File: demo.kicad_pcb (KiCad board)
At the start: 4 copper layers, 36 x 12.5 mm, 32 parts, among them J2 Conn_01x06, J3 Conn_01x04, J4 USB_C_Receptacle, U1 Regulator_Linear_XC6220B331MR, U2 MCU_ST_STM32F1_STM32F103C8Tx, Y2 8M

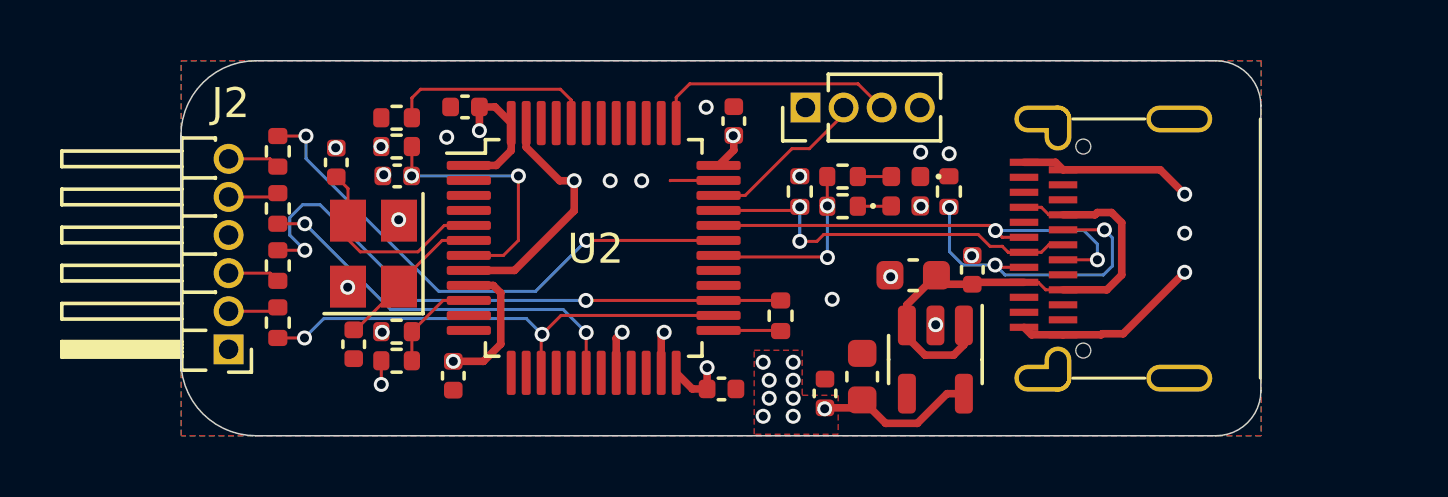
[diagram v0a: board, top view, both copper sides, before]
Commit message: update files
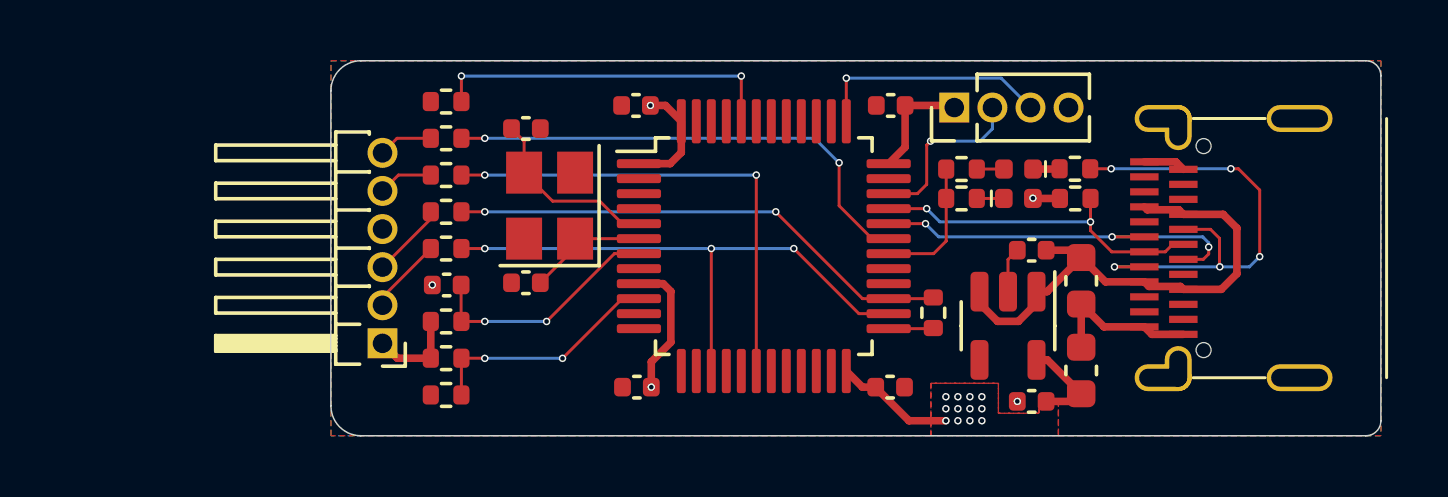
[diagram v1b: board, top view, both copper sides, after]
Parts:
- moved C5 17.0 mm to (118.6, 110.9), turned to 0 degrees
- moved C3 11.0 mm to (118.7, 101.5), turned to 180 degrees
- moved R8 9.18 mm to (124.8, 104.6), turned to 0 degrees
- moved C7 7.30 mm to (125.0, 110.3)
- moved C8 6.90 mm to (123.4, 111.4), turned to 180 degrees
- moved C10 6.42 mm to (106.5, 102.3), turned to 180 degrees
- moved C4 6.13 mm to (110.2, 110.9), turned to 180 degrees
- moved R4 6.13 mm to (103.8, 106.3), turned to 180 degrees
- moved C9 6.10 mm to (106.5, 107.4), turned to 0 degrees
- moved Y2 6.08 mm to (107.3, 104.8)
- moved R11 6.06 mm to (103.8, 108.7)
- moved R5 5.89 mm to (103.8, 105.0), turned to 180 degrees
- moved R6 5.72 mm to (103.8, 103.8), turned to 180 degrees
- moved U2 5.67 mm to (114.4, 106.2)
- moved R7 5.63 mm to (103.8, 102.6), turned to 180 degrees
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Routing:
- net GND: track 24.8 -> 9.06 mm, vias 21 -> 2
- net Net-(J4-CC1): track 11.0 -> 16.5 mm, vias 3 -> 5
- net +3V3: track 18.7 -> 23.5 mm, vias 17 -> 15
- net /BOOT0: track 7.01 -> 11.7 mm, vias 0 -> 2
- net Net-(U2-PA0): track 3.30 -> 7.97 mm, vias 0 -> 2
- net /T_NRST: track 13.1 -> 16.4 mm
- net /T_JTMS: track 20.1 -> 16.9 mm
- net /T_JTCK: track 16.7 -> 19.2 mm, vias 2 -> 3
- net /STLINK_USB_DM-: track 15.6 -> 13.3 mm, vias 2 -> 3
- net /LED_STLINK: track 6.37 -> 4.49 mm, vias 2 -> 0
- net /STLINK_USB_DP+: track 13.1 -> 11.5 mm
- net /SWO: track 18.0 -> 16.5 mm
- net Net-(U2-PD1): track 5.13 -> 4.08 mm
- net /SWCLK: track 1.69 -> 2.56 mm
- net /SWDIO: track 1.75 -> 2.51 mm
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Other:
- board size 36 x 12.5 mm -> 35 x 12.5 mm
- board text added: "3V3"
- board text added: "GND"
- board text added: "NRST"
- board text added: "SWCLK"
- board text added: "SWDIO"
- board text added: "SWO"
- board text added: "Type-C STLINK"
